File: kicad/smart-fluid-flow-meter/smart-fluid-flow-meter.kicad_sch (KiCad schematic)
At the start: 11 parts, among them J1 YF-S201, SW1 Factory reset button, U1 ESP32-WROOM-32

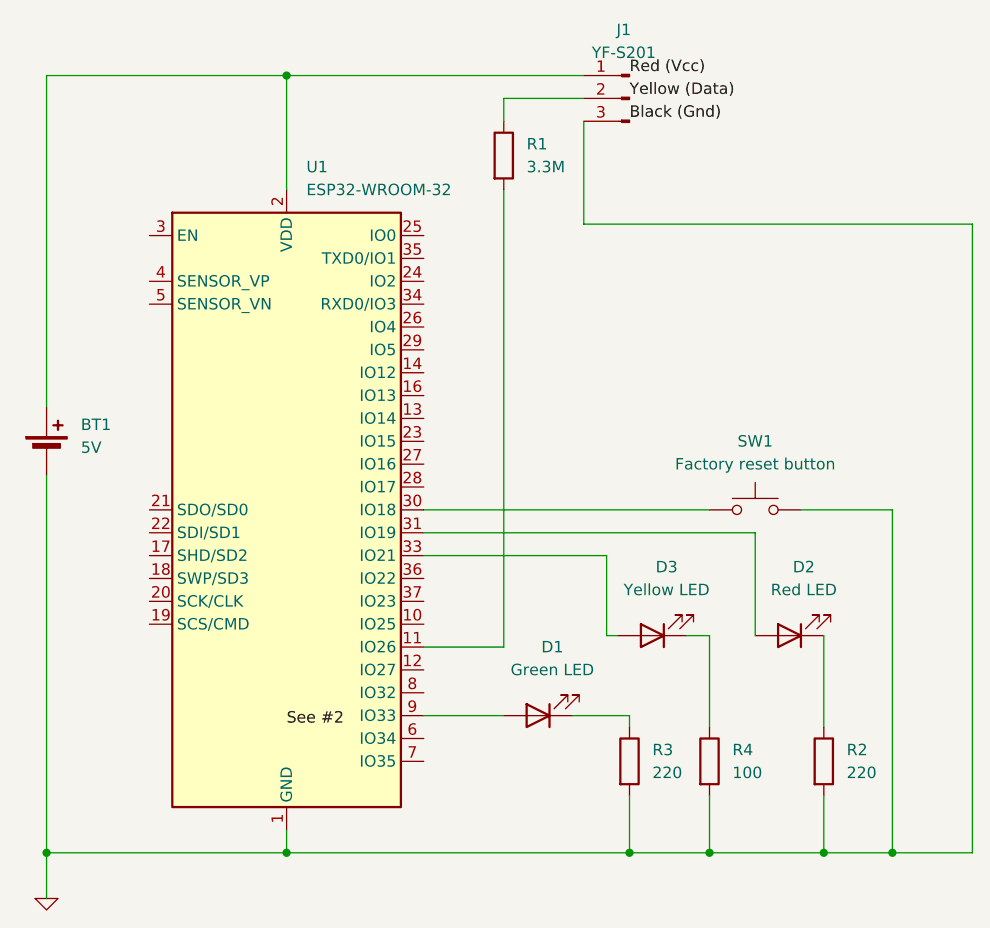
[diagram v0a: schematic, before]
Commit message: Design PCB (#74)
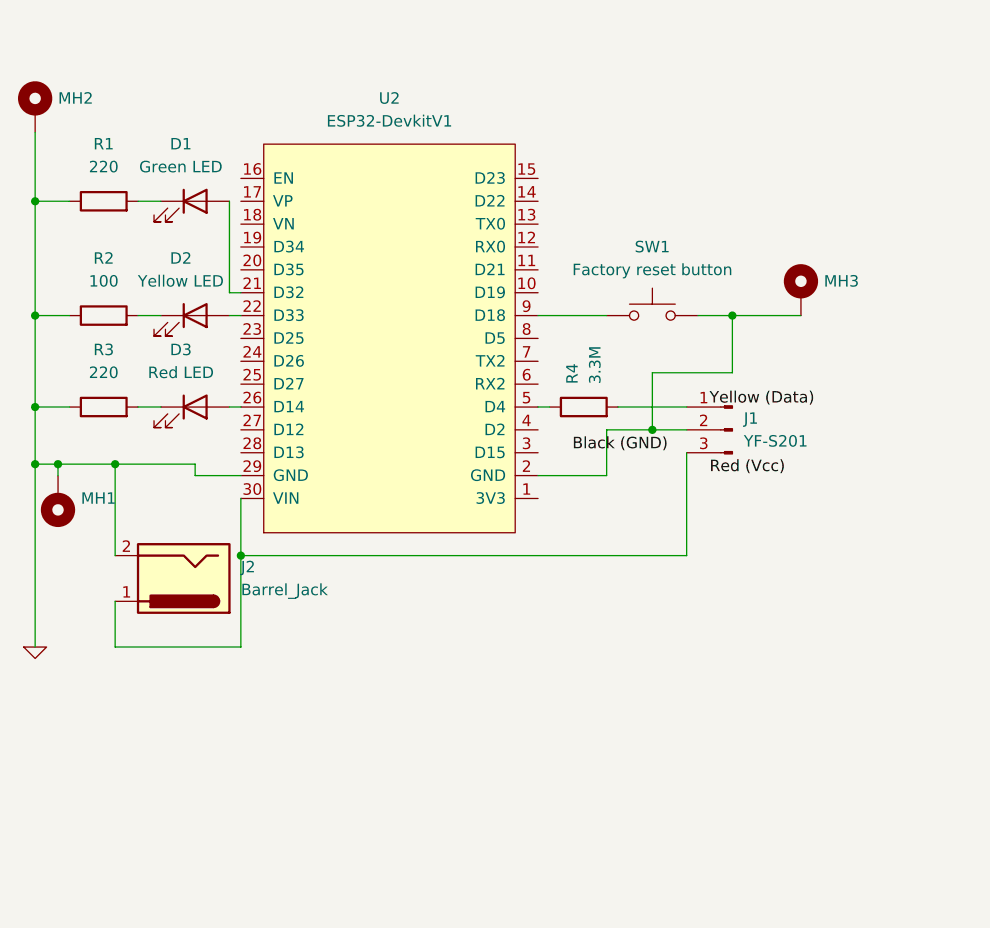
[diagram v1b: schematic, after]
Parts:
- removed BT1: 5V, symbol Device:Battery_Cell
- removed U1: ESP32-WROOM-32, RF_Module:ESP32-WROOM-32, symbol RF_Module:ESP32-WROOM-32
- added J2: Barrel_Jack, Connector_BarrelJack:BarrelJack_CUI_PJ-063AH_Horizontal, symbol Connector:Barrel_Jack
- added MH1, MH2, MH3: MountingHole_Pad, MountingHole:MountingHole_3.2mm_M3_Pad_Via, symbol Mechanical:MountingHole_Pad
- added U2: ESP32-DevkitV1, footprints:esp32_devkit_v1, symbol esp32-devkitv1:MyLib_ESP32_DEVKITV1
- D1: footprint (none) -> LED_THT:LED_D5.0mm
- D2: renamed from D3; footprint (none) -> LED_THT:LED_D5.0mm
- D3: renamed from D2; footprint (none) -> LED_THT:LED_D5.0mm
- J1: footprint (none) -> Connector_JST:JST_EH_B3B-EH-A_1x03_P2.50mm_Vertical
- R1: renamed from R3; footprint (none) -> Resistor_THT:R_Axial_DIN0207_L6.3mm_D2.5mm_P10.16mm_Horizontal
- R2: renamed from R4; footprint (none) -> Resistor_THT:R_Axial_DIN0207_L6.3mm_D2.5mm_P10.16mm_Horizontal
- R3: renamed from R2; footprint (none) -> Resistor_THT:R_Axial_DIN0207_L6.3mm_D2.5mm_P10.16mm_Horizontal
- R4: renamed from R1; footprint (none) -> Resistor_THT:R_Axial_DIN0207_L6.3mm_D2.5mm_P10.16mm_Horizontal
- SW1: footprint (none) -> Button_Switch_THT:SW_PUSH_1P1T_6x3.5mm_H4.3_APEM_MJTP1243
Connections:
- net 0: now also R1.1, R2.1, R3.1, J2.2, MH1.1, MH2.1, U2.29 (GND); no longer J1.3 (Pin_3), R1.2, R2.2, R3.2, SW1.2
- net at R4.2: now also J1.1 (Pin_1)
- net at SW1.1: now also U2.9 (D18)
- net at D3.2 (A): now also U2.26 (D14)
- net at D2.2 (A): now also U2.22 (D33)
- net at D1.2 (A): now also U2.21 (D32)
- net at D2.1 (K): now also R2.2; no longer R2.1
- net at D1.1 (K): now also R1.2; no longer R1.1
- net at D3.1 (K): now also R3.2; no longer R3.1
- net at J1.2 (Pin_2): now also SW1.2, MH3.1, U2.2 (GND); no longer R4.1
- new net: J1.3 (Pin_3), J2.1, U2.30 (VIN)
- new net: R4.1, U2.5 (D4)
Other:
- moved on the sheet: D1, D2, D3, J1, R1, R2, R3, R4, SW1
